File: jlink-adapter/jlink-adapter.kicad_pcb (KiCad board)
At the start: 2 copper layers, 52.7 x 30.2 mm, 21 parts, among them J1 USB_C_Receptacle_USB2.0, J2 Conn_ARM_JTAG_SWD_20, J3 ESPProgJTAG_TX, J4 Conn_01x05, J5 Conn_01x06, J6 USB_A, U1 USBLC6-2SC6, U2 XC6209, U3 USBLC6-2SC6, U4 USBLC6-2SC6, U5 USBLC6-2SC6

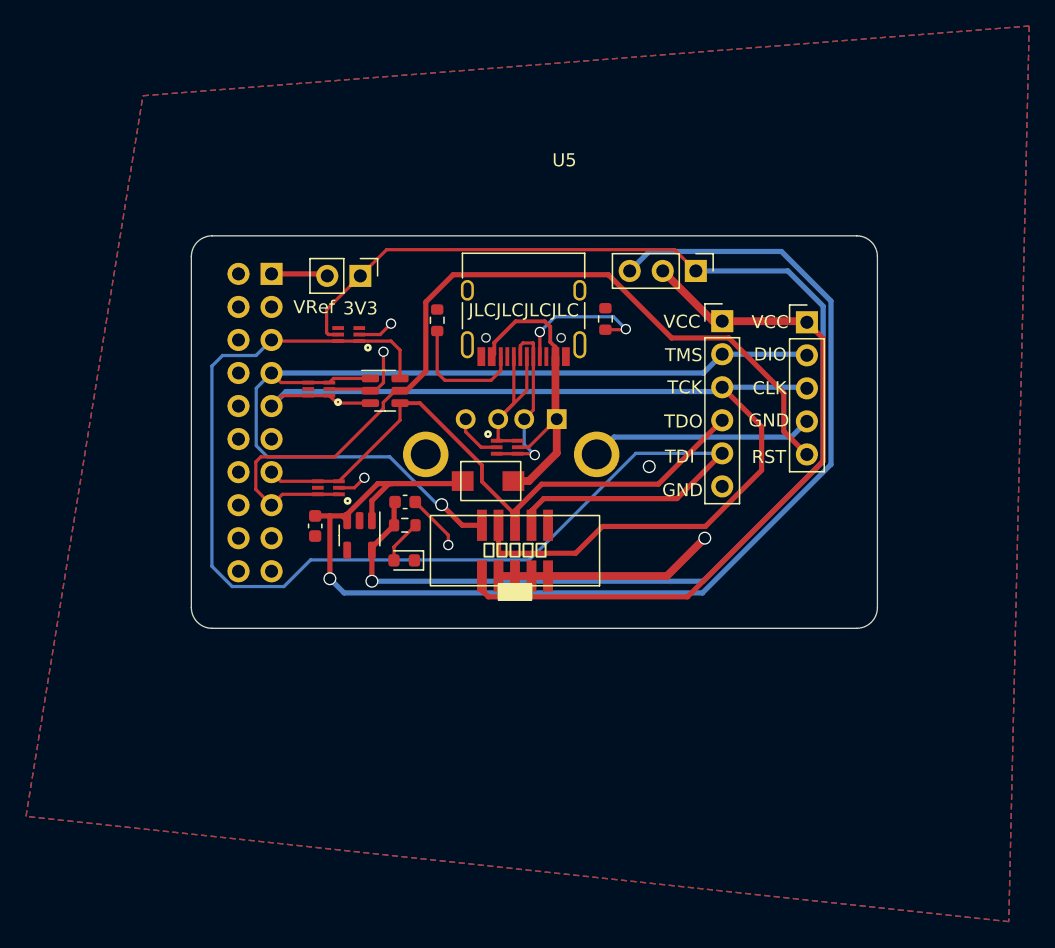
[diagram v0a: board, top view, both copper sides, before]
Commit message: 预备投板
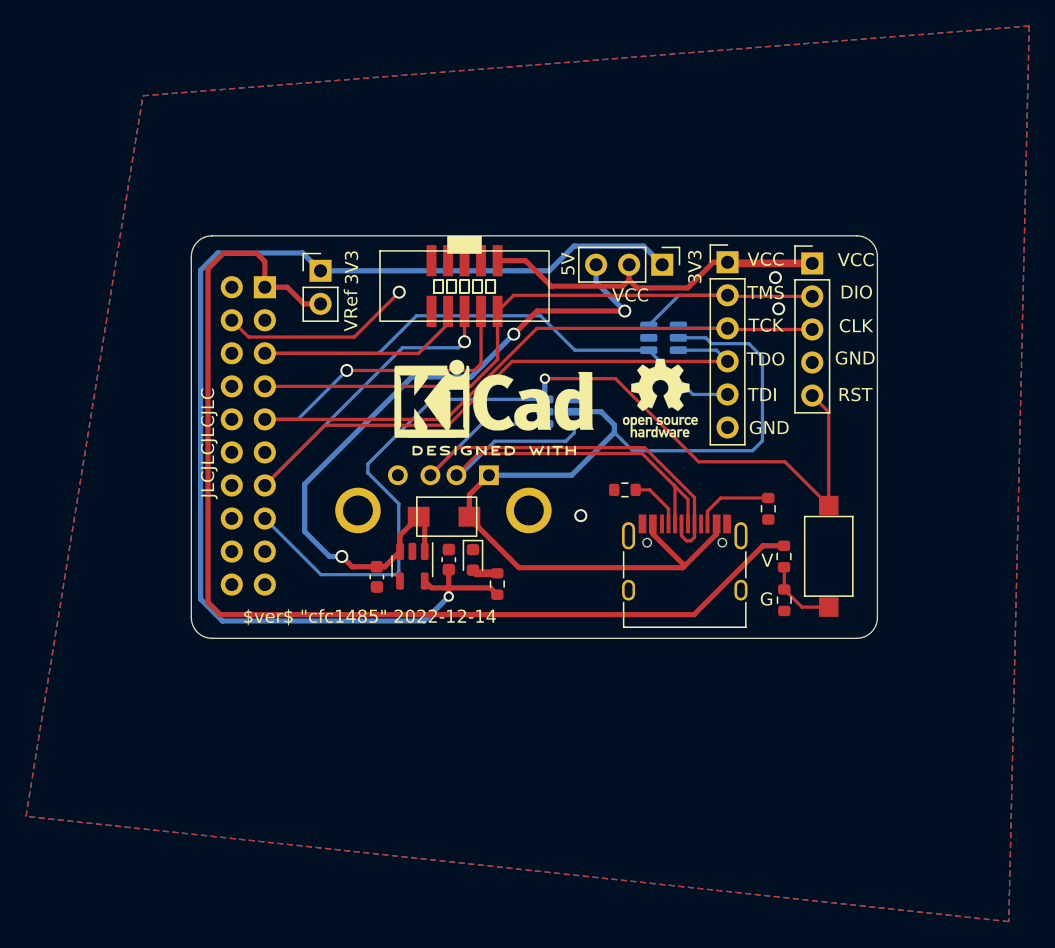
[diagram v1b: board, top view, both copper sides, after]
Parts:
- removed D2: SMS05CT1G, Package_TO_SOT_SMD:SOT-23-6
- removed U1, U4: USBLC6-2SC6, KisonCommon:USBLC6-2P6-SOT666
- added R1: 0, Resistor_SMD:R_0603_1608Metric, F.Cu at (188.0, 127.1)
- added R4: 0, Resistor_SMD:R_0603_1608Metric, F.Cu at (188.0, 123.7)
- added REF**: KiCad-Logo2_6mm_SilkScreen, Symbol:KiCad-Logo2_6mm_SilkScreen, F.Cu at (165.7, 111.6)
- added REF**: OSHW-Logo_5.7x6mm_SilkScreen, Symbol:OSHW-Logo_5.7x6mm_SilkScreen, F.Cu at (178.5, 111.5)
- added SW1: SW_Push, Button_Switch_SMD:SW_SPST_CK_RS282G05A3, F.Cu at (191.4, 123.7)
- U3, U5: value USBLC6-2SC6 -> USBLC6-4SC6; footprint KisonCommon:USBLC6-2P6-SOT666 -> Package_TO_SOT_SMD:SOT-23-6; moved to B.Cu
- moved R3 29.3 mm to (186.8, 120.0), turned to 90 degrees
- moved U3 26.7 mm to (178.7, 106.9)
- moved J1 24.3 mm to (180.3, 125.2), turned to 0 degrees
- moved J3 20.7 mm to (163.4, 102.9), turned to 0 degrees
- moved R2 13.2 mm to (175.8, 118.6), turned to 0 degrees
- moved R6 8.42 mm to (165.9, 125.8), turned to 90 degrees
- moved U5 7.32 mm to (170.7, 112.6), turned to 0 degrees
- moved J6 6.76 mm to (165.3, 117.5)
- moved C1 6.15 mm to (156.7, 125.3)
- moved C2 5.56 mm to (162.2, 124.0), turned to 90 degrees
- moved D3 5.29 mm to (164.1, 124.0), turned to -90 degrees
- moved U2 4.70 mm to (159.4, 124.5)
- moved J5 4.55 mm to (183.6, 101.1)
- moved J4 4.55 mm to (190.2, 101.2)
- moved D1 4.36 mm to (162.1, 120.7)
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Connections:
- U3 pad 1: /SRST -> /TDI
- U3 pad 3: /TDO -> /SWDIO
- U3 pad 4: /TDO -> /SWDCLK
- U3 pad 5: unconnected-(U3-Pad5) -> VBUS
- U3 pad 6: /SRST -> /TDO
- U5 pad 3: /DN -> /SRST
- U5 pad 4: /DN -> unconnected-(U5-Pad4)
- U5 pad 6: /DP -> /DN
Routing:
- net /VREF: track 4.35 -> 84.4 mm
- net VBUS: track 25.1 -> 71.5 mm
- net /EXT_5V: track 94.8 -> 53.3 mm, vias 1 -> 3
- net /TDI: track 94.9 -> 55.2 mm
- net GND: track 54.5 -> 14.8 mm, vias 6 -> 4
- net /DeviceVcc: track 55.8 -> 27.5 mm
- net /DP: track 14.3 -> 38.4 mm
- net /DN: track 14.1 -> 36.0 mm, vias 1 -> 0
- net /SWDIO: track 75.8 -> 54.2 mm, vias 1 -> 0
- net /TDO: track 47.3 -> 65.9 mm, vias 0 -> 1
- net /SWDCLK: track 82.6 -> 71.3 mm, vias 0 -> 1
- net +3V3: track 101.9 -> 91.9 mm
- net Net-(J1-PadA5): track 11.0 -> 4.29 mm, vias 2 -> 0
- net Net-(SW1-Pad2): track 0.00 -> 5.70 mm
- net /SRST: track 68.5 -> 73.6 mm, vias 0 -> 1
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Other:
- board size 52.7 x 30.2 mm -> 52.7 x 30.9 mm
- board text added: "$ver$ "cfc1485" 2022-12-14"
- board text added: "5V"
- board text added: "G"
- board text added: "V"
